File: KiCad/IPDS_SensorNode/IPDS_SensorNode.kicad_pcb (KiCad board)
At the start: 2 copper layers, 120 x 90 mm, 18 parts, among them J1 ESP32_Left, J2 ESP32_Right, J3 MPU6050, J4 DS3231_RTC, J5 NEO-6M_GPS, J6 USB_Micro_B

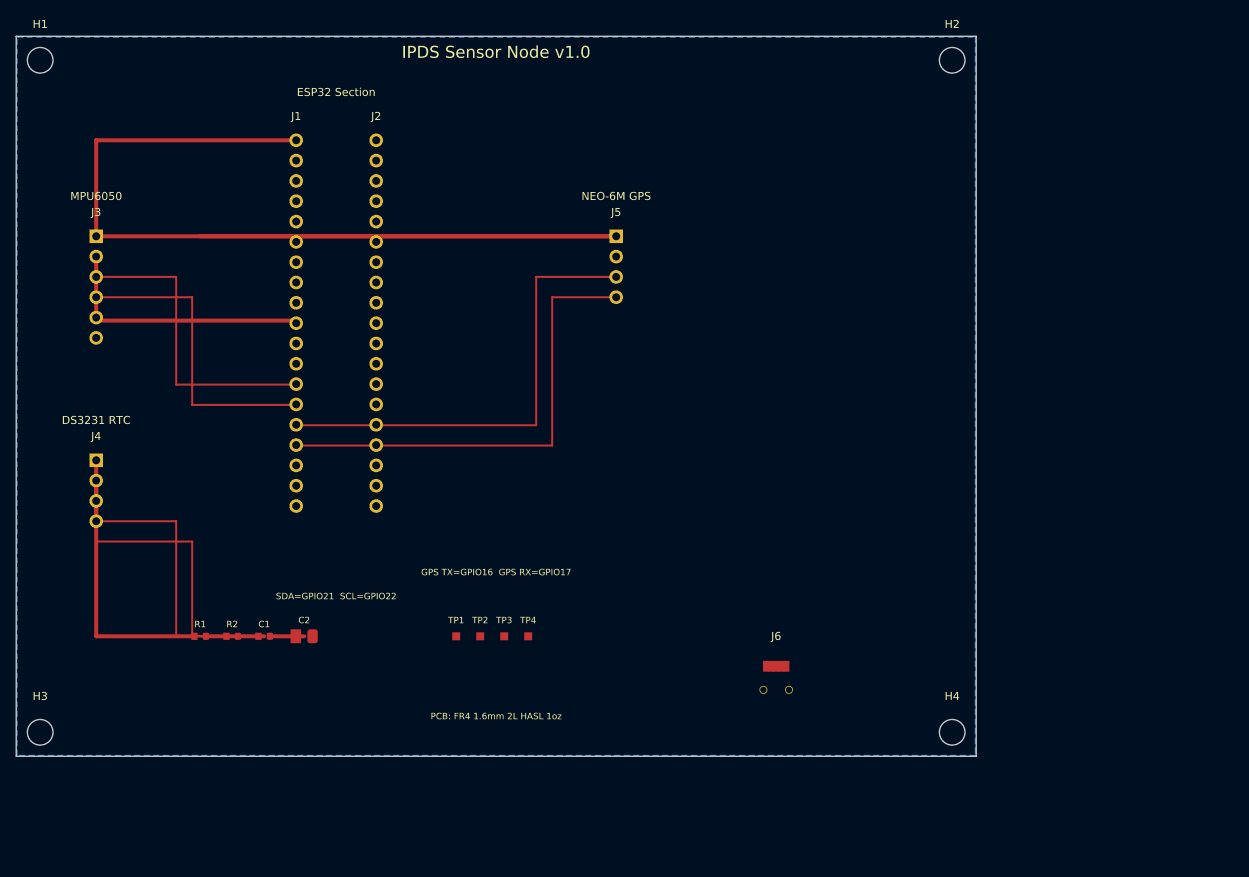
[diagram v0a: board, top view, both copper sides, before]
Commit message: Update KiCad sensor node PCB layout, symbol libraries, and fabrication outputs
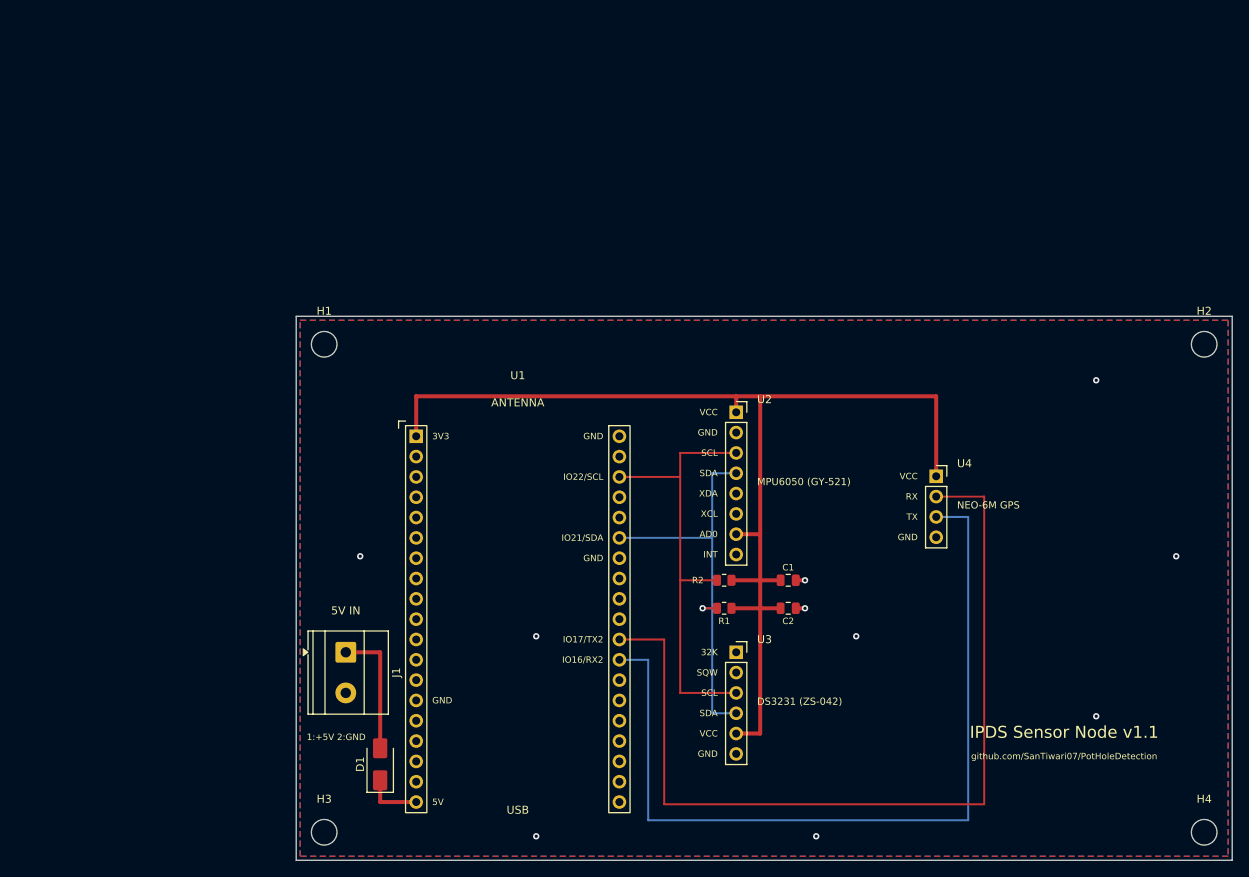
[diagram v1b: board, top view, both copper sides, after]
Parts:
- removed J2: ESP32_Right, Connector_PinHeader_2.54mm:PinHeader_1x19_P2.54mm_Vertical
- removed J3: MPU6050, Connector_PinHeader_2.54mm:PinHeader_1x06_P2.54mm_Vertical
- removed J4: DS3231_RTC, Connector_PinHeader_2.54mm:PinHeader_1x04_P2.54mm_Vertical
- removed J5: NEO-6M_GPS, Connector_PinHeader_2.54mm:PinHeader_1x04_P2.54mm_Vertical
- removed J6: USB_Micro_B, Connector_USB:USB_Micro-B_Molex_47589-0001
- removed TP1: +3V3, TestPoint:TestPoint_Pad_1.0x1.0mm
- removed TP2: GND, TestPoint:TestPoint_Pad_1.0x1.0mm
- removed TP3: SDA, TestPoint:TestPoint_Pad_1.0x1.0mm
- removed TP4: SCL, TestPoint:TestPoint_Pad_1.0x1.0mm
- added D1: SS14, Diode_SMD:D_SMA, F.Cu at (50.5, 96.0)
- added U1: ESP32-DevKitC_38pin, IPDS:ESP32_DevKitC_38_Socket, F.Cu at (55.0, 55.0)
- added U2: GY-521_MPU6050, Connector_PinSocket_2.54mm:PinSocket_1x08_P2.54mm_Vertical, F.Cu at (95.0, 52.0)
- added U3: ZS-042_DS3231, Connector_PinSocket_2.54mm:PinSocket_1x06_P2.54mm_Vertical, F.Cu at (95.0, 82.0)
- added U4: GY-NEO6MV2, Connector_PinSocket_2.54mm:PinSocket_1x04_P2.54mm_Vertical, F.Cu at (120.0, 60.0)
- C1: footprint Capacitor_SMD:C_0402_1005Metric -> Capacitor_SMD:C_0805_2012Metric
- H1, H2, H3, H4: value MountingHole_3.2mm_M3 -> M3
- J1: value ESP32_Left -> 5V_IN; footprint Connector_PinHeader_2.54mm:PinHeader_1x19_P2.54mm_Vertical -> TerminalBlock_Phoenix:TerminalBlock_Phoenix_MKDS-1,5-2-5.08_1x02_P5.08mm_Horizontal
- R1, R2: footprint Resistor_SMD:R_0402_1005Metric -> Resistor_SMD:R_0805_2012Metric
- moved C1 65.9 mm to (101.5, 73.0)
- moved R1 65.6 mm to (93.5, 76.5), turned to 180 degrees
- moved J1 64.3 mm to (46.2, 82.0), turned to -90 degrees
- moved R2 61.9 mm to (93.5, 73.0), turned to 180 degrees
- moved C2 60.6 mm to (101.5, 76.5)
- moved H1 50.2 mm to (43.5, 43.5)
- moved H2 47.5 mm to (153.5, 43.5)
- moved H3 37.6 mm to (43.5, 104.5)
- moved H4 33.9 mm to (153.5, 104.5)
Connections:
- J1 pad 1: +3V3 -> /VIN_EXT
- J1 pad 2: (no net) -> GND
- R1 pad 2: SDA -> /SDA
- R2 pad 2: SCL -> /SCL
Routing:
- net /ESP_TX2: track 0.00 -> 110.7 mm
- net /ESP_RX2: track 0.00 -> 105.6 mm
- net SCL: track 68.0 -> 0.00 mm
- net SDA: track 66.6 -> 0.00 mm
- net GPS_TX: track 58.5 -> 0.00 mm
- net GPS_RX: track 58.5 -> 0.00 mm
- net /SCL: track 0.00 -> 56.2 mm
- net /SDA: track 0.00 -> 50.6 mm, vias 0 -> 1
- net GND: track 48.5 -> 2.30 mm, vias 0 -> 10
- net +3V3: track 188.3 -> 142.4 mm
- net /VIN_EXT: track 0.00 -> 16.3 mm
- net +5V: track 0.00 -> 7.22 mm
- added copper zone on F.Cu, net GND
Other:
- board size 120 x 90 mm -> 117 x 68 mm
- rule pad_to_mask_clearance: 0.05 -> 0
- board text added: "1:+5V 2:GND"
- board text added: "32K"
- board text added: "5V IN"
- board text added: "AD0"
- board text added: "DS3231 (ZS-042)"
- board text added: "GND"
- board text added: "INT"
- board text added: "IPDS Sensor Node v1.1"
- board text added: "MPU6050 (GY-521)"
- board text added: "RX"
- board text added: "SCL"
- board text added: "SDA"
- board text added: "SQW"
- board text added: "TX"
- board text added: "VCC"
- board text added: "XCL"
- board text added: "XDA"
- board text added: "github.com/SanTiwari07/PotHoleDetection"
- board text removed: "DS3231 RTC"
- board text removed: "ESP32 Section"
- board text removed: "GPS TX=GPIO16 GPS RX=GPIO17"
- board text removed: "IPDS Sensor Node v1.0"
- board text removed: "MPU6050"
- board text removed: "PCB: FR4 1.6mm 2L HASL 1oz"
- board text removed: "SDA=GPIO21 SCL=GPIO22"
